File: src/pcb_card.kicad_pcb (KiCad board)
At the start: 2 copper layers, 72.4 x 41.2 mm, 137 parts, among them J1 UART, J2 SOICbite, SW1 TS-1187A-B-A-B, SW2 TS-1187A-B-A-B, U1 CH32V003FxUx, U2 LIS3DH, U3 CH32X035F8U6_C42442062

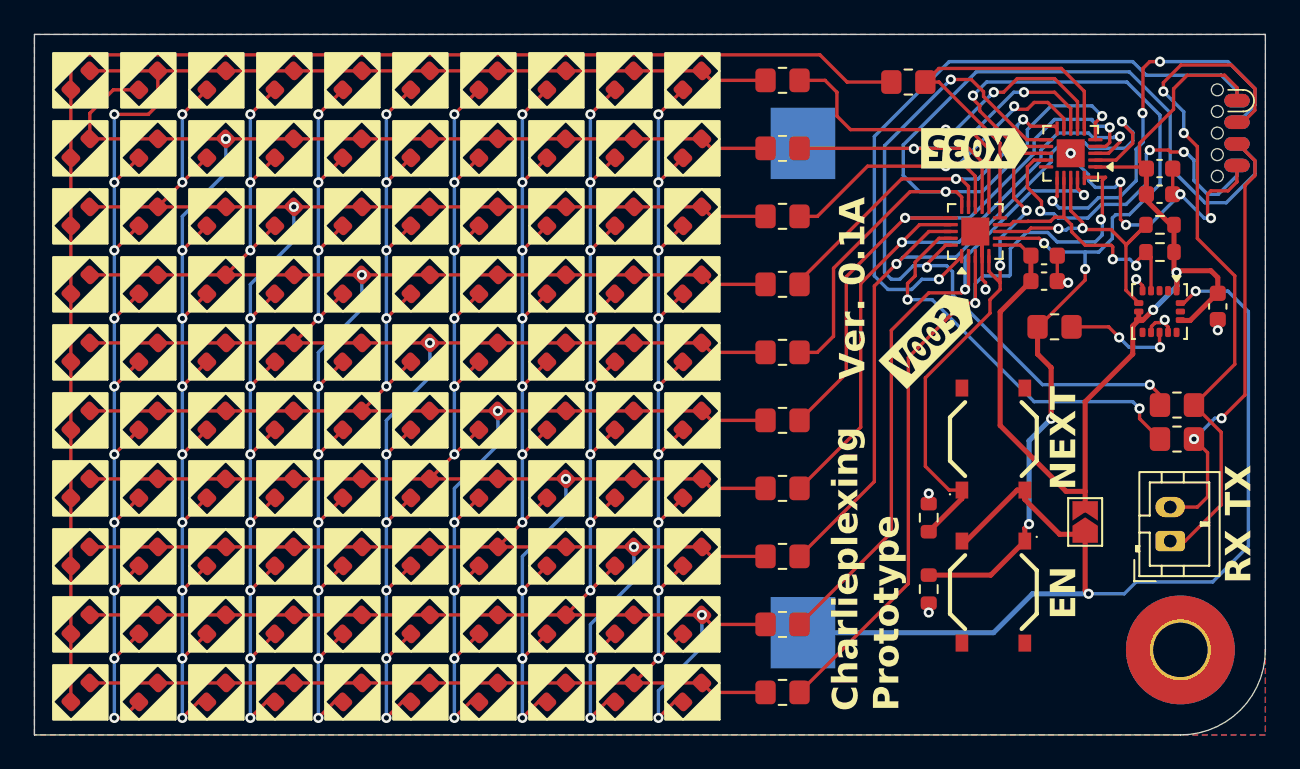
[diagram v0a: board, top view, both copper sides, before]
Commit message: chore: breaks out I2C pins
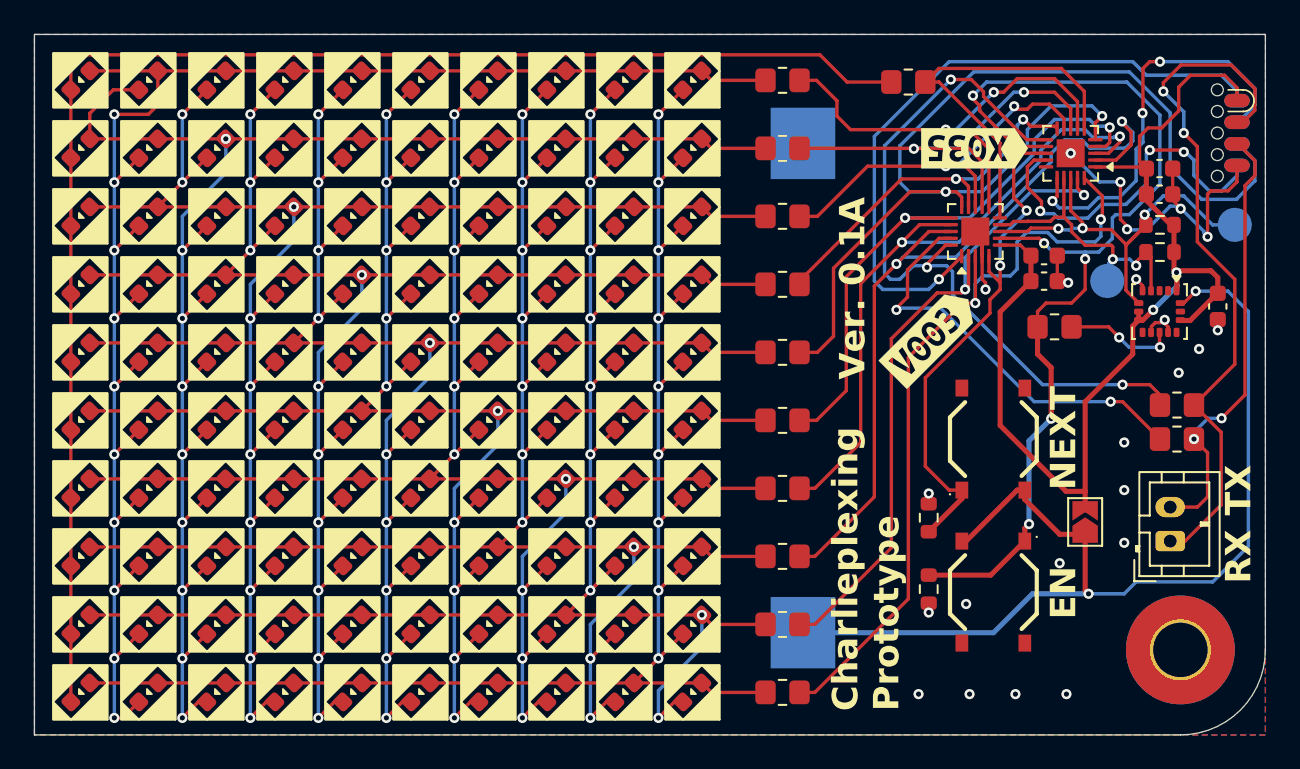
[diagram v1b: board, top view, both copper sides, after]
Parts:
- added TP1: SCL, TestPoint:TestPoint_Pad_D2.0mm, B.Cu at (167.1, 118.5)
- added TP2: SDA, TestPoint:TestPoint_Pad_D2.0mm, B.Cu at (174.6, 115.2)
- added kibuzzard-6A30280D: G***, kibuzzard-6A30280D, B.Cu at (174.7, 119.3)
- added kibuzzard-6A302872: G***, kibuzzard-6A302872, B.Cu at (164.4, 121.6)
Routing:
- net SDA: track 18.3 -> 25.3 mm, vias 2 -> 3
- net SCL: track 15.8 -> 17.7 mm
- net GND: track 30.7 -> 31.8 mm, vias 12 -> 23
- net TX: track 23.7 -> 24.7 mm
- net EN: track 59.7 -> 60.7 mm
- net CH_4: track 38.3 -> 39.0 mm
- net CH_6: track 65.3 -> 66.0 mm
- net CH_3: track 46.5 -> 47.1 mm
- net CH_5: track 34.2 -> 34.7 mm
